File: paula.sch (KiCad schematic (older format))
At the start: 79 parts, among them CN200 DB9P RIGHT(1), CN201 DB9P LEFT(0), CN204 RIGHT AUDIO, CN205 LEFT AUDIO, J200 Conn_01x03_Male, Q200 MPF102, Q201 MPF102, Q202 2N3906, U200 PAULA, U202 74LS157, U204 LF347

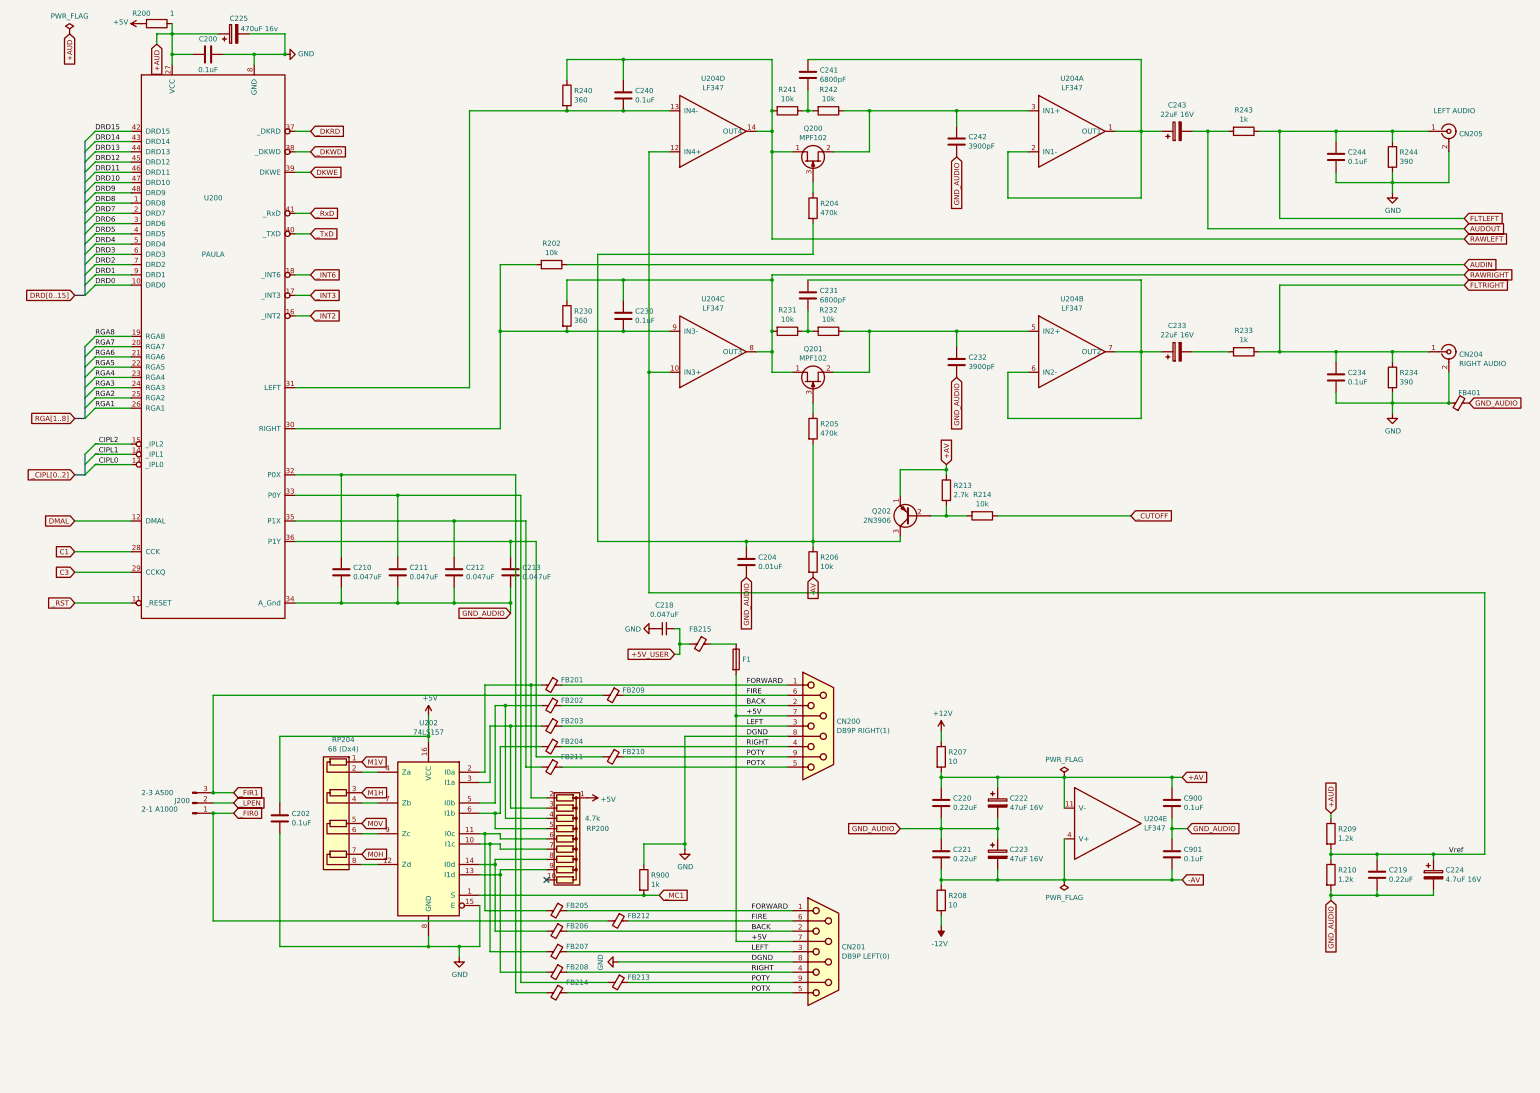
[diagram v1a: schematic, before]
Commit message: Review started; oopsie whoopsie
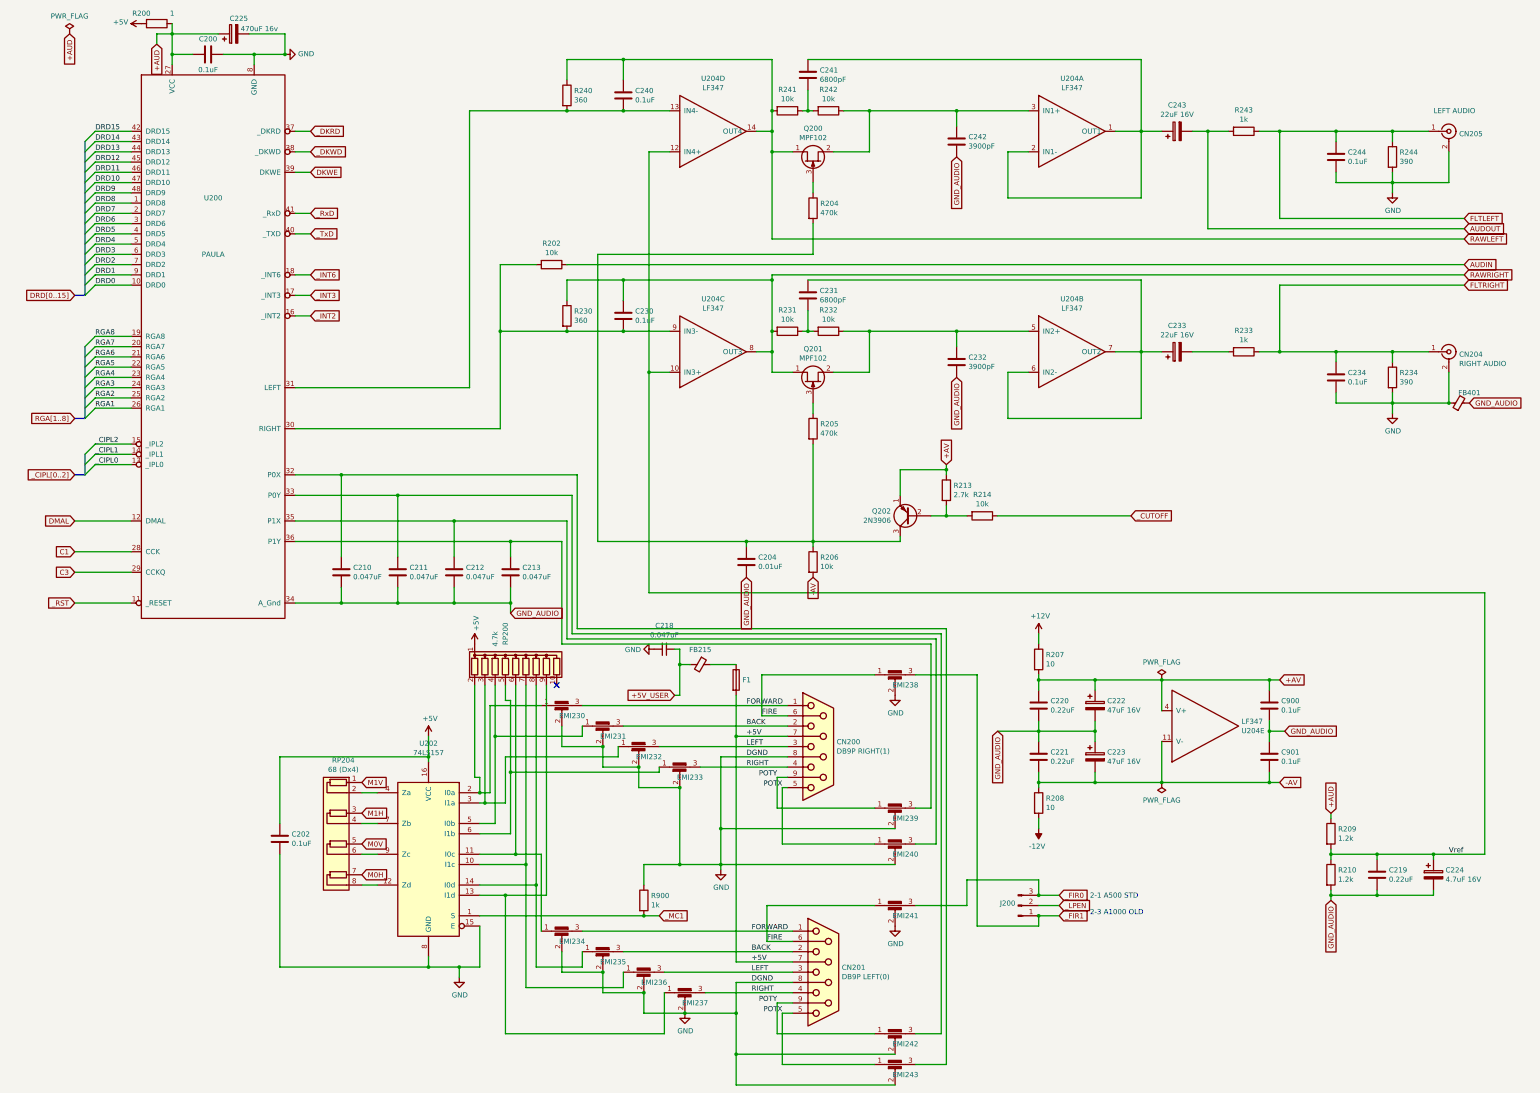
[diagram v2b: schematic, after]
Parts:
- removed FB201, FB202, FB203, FB204, FB205, FB206, FB207, FB208, FB209, FB210, FB211, FB212, FB213, FB214: Ferrite_Bead_Small, symbol Device:Ferrite_Bead_Small
- added EMI230, EMI231, EMI232, EMI233, EMI234, EMI235, EMI236, EMI237, EMI238, EMI239, EMI240, EMI241, EMI242, EMI243: C_Feedthrough, symbol Device:C_Feedthrough
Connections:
- net +AV: now also U204.4 (V+); no longer U204.11 (V-)
- net -AV: now also U204.11 (V-); no longer U204.4 (V+)
- net BACK: now also EMI231.3, EMI235.3
- net FIRE: now also EMI238.1, EMI241.1
- net FORWARD: now also EMI230.3, EMI234.3
- net GND: now also EMI230.2, EMI231.2, EMI232.2, EMI233.2, EMI234.2, EMI235.2, EMI236.2, EMI237.2, EMI238.2, EMI239.2, EMI240.2, EMI241.2, EMI242.2, EMI243.2
- net LEFT: now also EMI232.3, EMI236.3
- net POTX: now also EMI240.1, EMI243.1
- net POTY: now also EMI239.1, EMI242.1
- net RIGHT: now also EMI233.3, EMI237.3
- net _FIR0: now also J200.3 (Pin_3), EMI241.3; no longer J200.1 (Pin_1)
- net _FIR1: now also J200.1 (Pin_1), EMI238.3; no longer J200.3 (Pin_3)
- net at C210.1, U200.32 (P0X): now also EMI243.3
- net at C211.1, U200.33 (P0Y): now also EMI242.3
- net at C212.1, U200.35 (P1X): now also EMI240.3
- net at C213.1, U200.36 (P1Y): now also EMI239.3
- net at RP200.7 (R6), U202.10 (I1c): now also EMI236.1
- net at RP200.6 (R5), U202.11 (I0c): now also EMI234.1
- net at RP200.9 (R8), U202.13 (I1d): now also EMI237.1
- net at RP200.8 (R7), U202.14 (I0d): now also EMI235.1
- net at RP200.2 (R1), U202.2 (I0a): now also EMI230.1
- net at RP200.3 (R2), U202.3 (I1a): now also EMI232.1
- net at RP200.4 (R3), U202.5 (I0b): now also EMI231.1
- net at RP200.5 (R4), U202.6 (I1b): now also EMI233.1
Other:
- note added: "2-1 A500 STD\n\n2-3 A1000 OLD"
- note removed: "2-3 A500\n\n2-1 A1000"
- moved on the sheet: C202, C218, C220, C221, C222, C223, C900, C901, CN200, CN201, F1, FB215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
